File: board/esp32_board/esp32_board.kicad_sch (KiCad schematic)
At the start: 14 parts, among them J1 Screw_Terminal_01x19, J2 Screw_Terminal_01x19, J3 Conn_01x19_Socket, J4 Conn_01x19_Pin, J5 Conn_01x19_Socket, J6 Conn_01x19_Pin, U1 ESP32-DevKitC

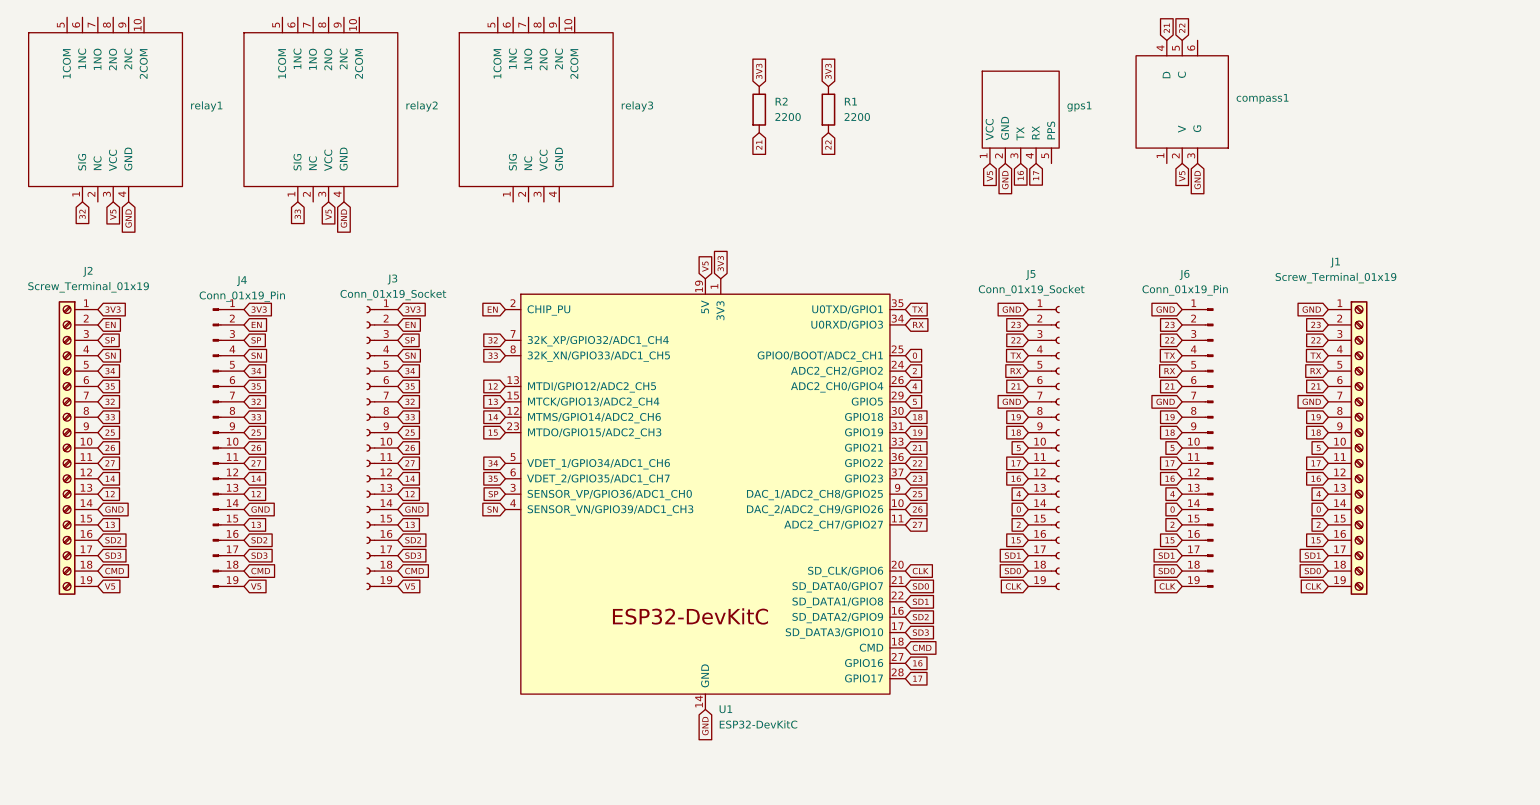
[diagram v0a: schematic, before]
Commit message: feat: Updated docs and board
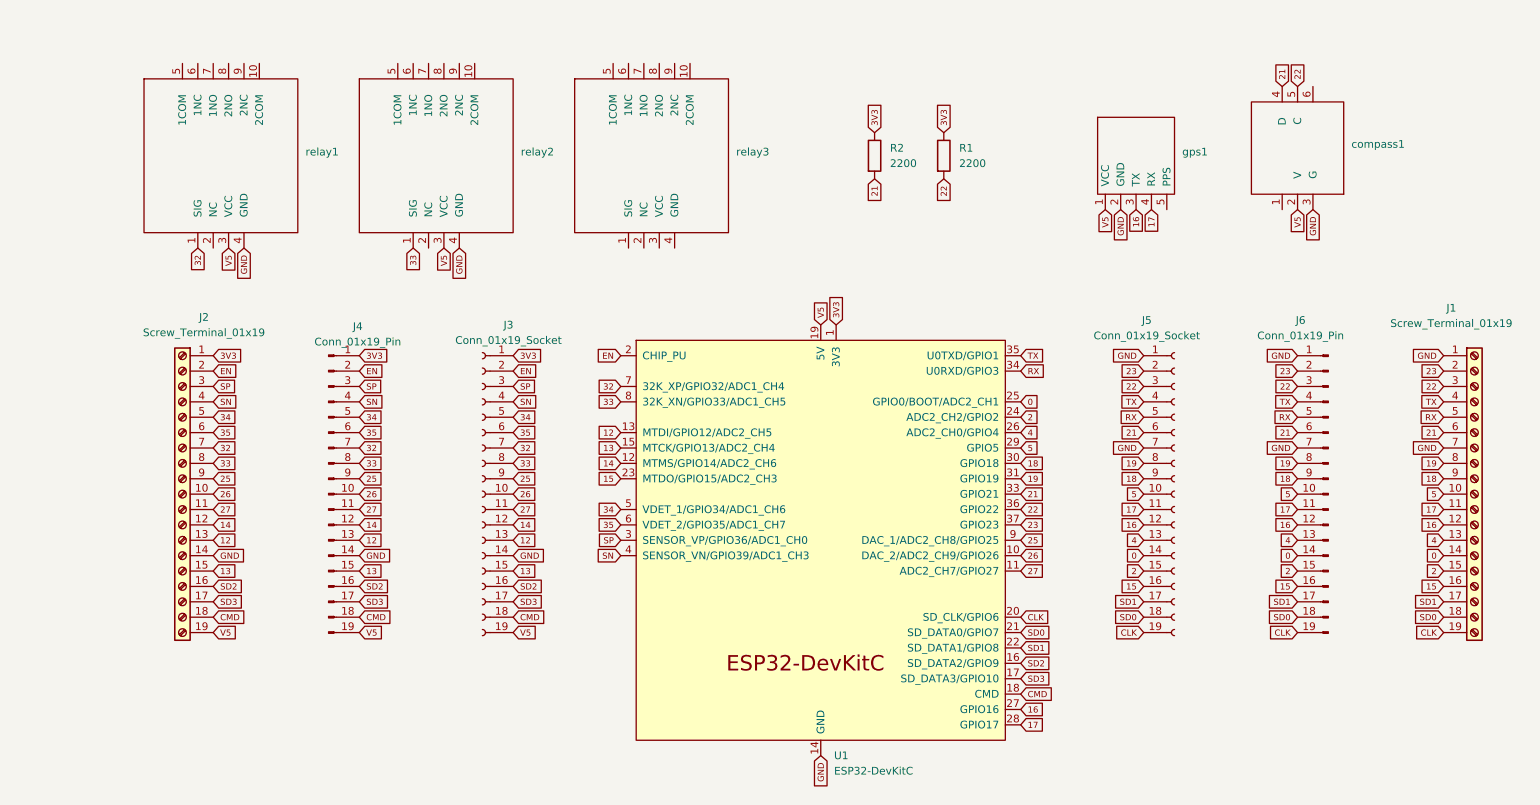
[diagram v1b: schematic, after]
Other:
- title: (none) -> Принципиальная схема
- moved on the sheet: J1, J2, J3, J4, J5, J6, R1, R2, U1, compass1, gps1, relay1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
